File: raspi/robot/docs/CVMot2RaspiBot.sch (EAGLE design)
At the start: 2 parts

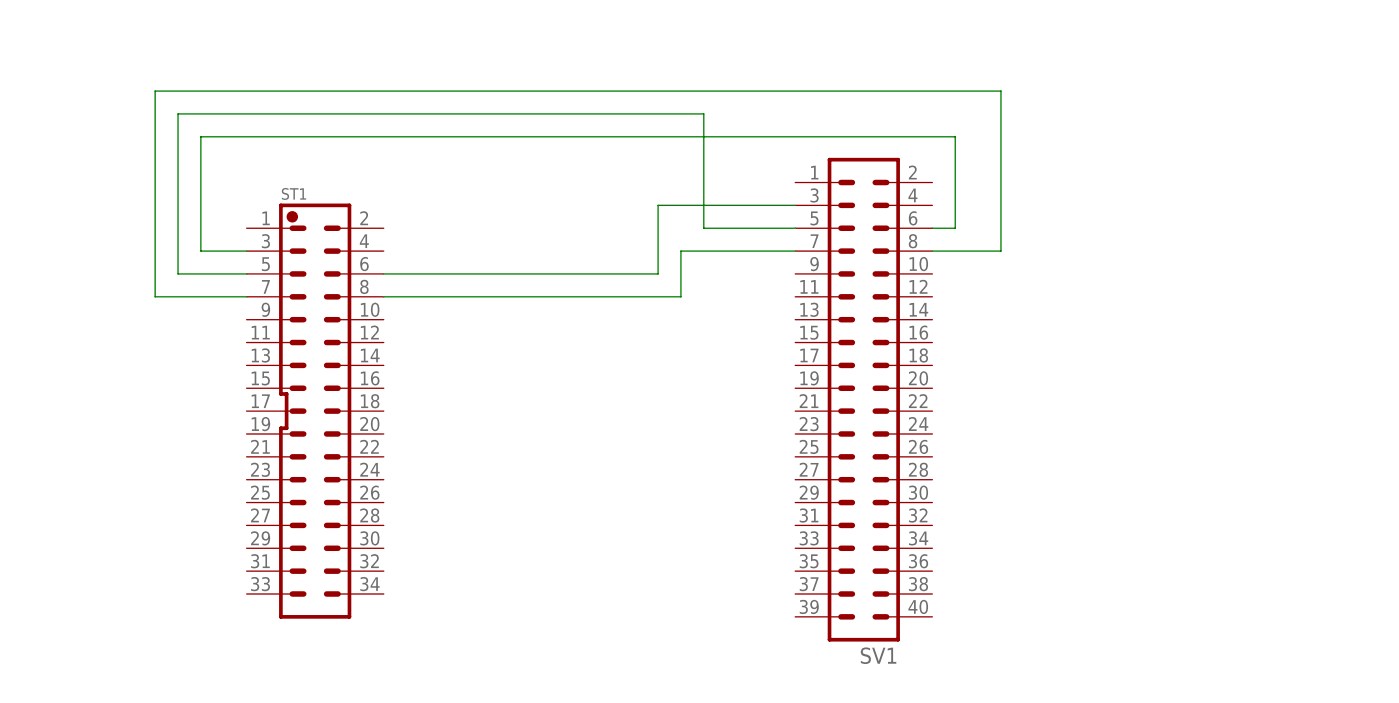
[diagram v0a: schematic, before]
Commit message: Raspi: Update Schaltpläne
git-svn-id: https://cvsvn/svn/raspi/trunk@93 50237d99-7d21-444e-87dd-016511c29f8c
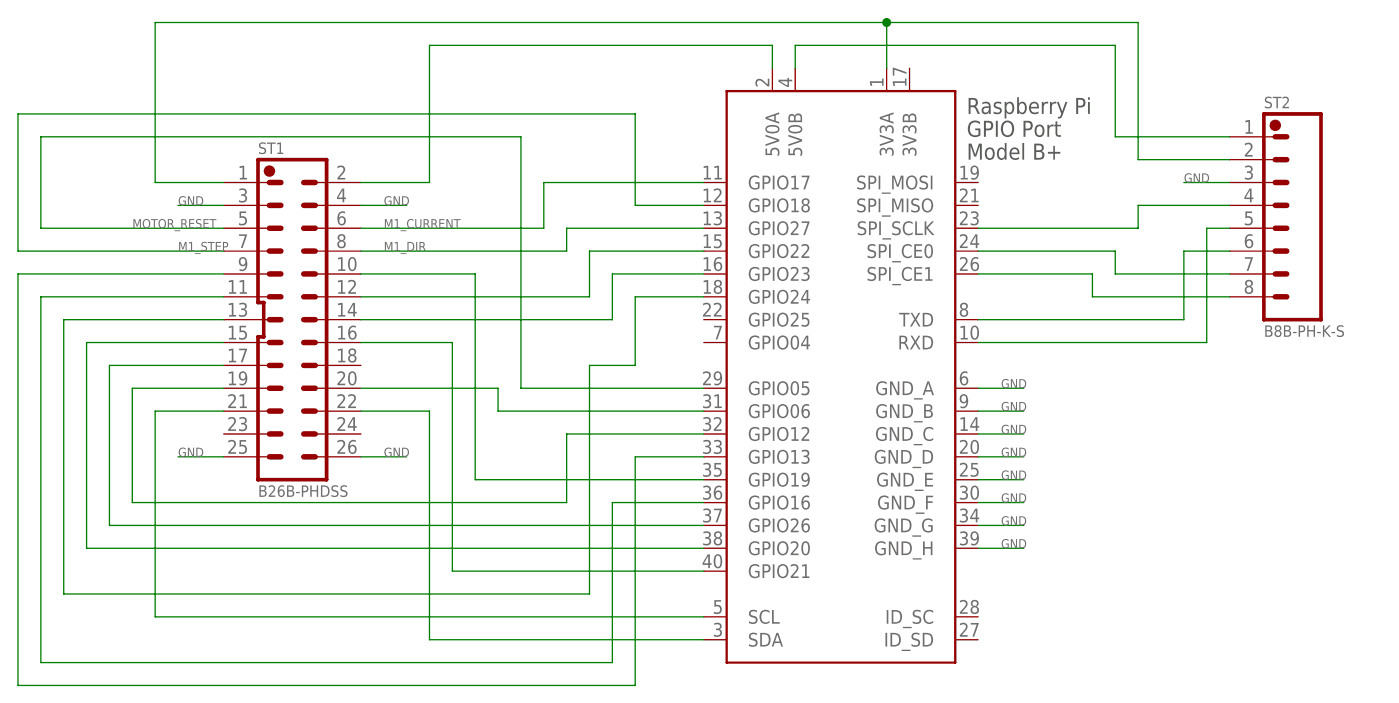
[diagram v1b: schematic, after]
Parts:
- removed SV1: (no value), con-harting-ml:ML40
- added ST2: B8B-PH-K-S, CV_Con:STK-08-1RJST-PH_8_TH
- added X1: RASPI_GPIO_B+#_PIN, raspberrypi_bastelstube_v13:RASPI_GPIO_B+#_PIN
- ST1: value (none) -> B26B-PHDSS; device CV_Con:STK-34-2R-MJST-PHD_34_TH -> CV_Con:STK-26-2RJST-PHD_26_TH
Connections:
- new net GND: ST1.25, ST1.26, ST1.3, ST1.4, ST2.3, X1.GND_A, X1.GND_B, X1.GND_C, X1.GND_D, X1.GND_E, X1.GND_F, X1.GND_G, X1.GND_H
- new net M1_CURRENT: ST1.6, X1.GPIO17
- new net M1_DIR: ST1.8, X1.GPIO27
- new net M1_STEP: ST1.7, X1.GPIO18
- new net MOTOR_RESET: ST1.5, X1.GPIO05
- new net N$10: ST1.19, X1.GPIO12
- new net N$11: ST1.20, X1.GPIO06
- new net N$19: ST2.4, X1.SPI_SCLK
- new net N$20: ST1.2, X1.5V0A
- new net N$21: ST1.1, ST2.2, X1.3V3A
- new net N$22: ST1.21, X1.SCL
- new net N$23: ST1.22, X1.SDA
- new net N$24: ST2.1, X1.5V0B
- new net N$27: ST2.5, X1.RXD
- new net N$28: ST2.6, X1.TXD
- new net N$29: ST2.7, X1.SPI_CE0
- new net N$30: ST2.8, X1.SPI_CE1
- new net N$6: ST1.13, X1.GPIO24
- new net N$7: ST1.15, X1.GPIO20
- new net N$8: ST1.17, X1.GPIO26
- new net N$9: ST1.16, X1.GPIO21
- net N$1: now also ST1.9, X1.GPIO13; no longer ST1.5, SV1.5
- net N$2: now also ST1.11, X1.GPIO16; no longer ST1.6, SV1.3
- net N$3: now also ST1.10, X1.GPIO19; no longer ST1.8, SV1.7
- net N$4: now also ST1.12, X1.GPIO22; no longer ST1.7, SV1.8
- net N$5: now also ST1.14, X1.GPIO23; no longer ST1.3, SV1.6
